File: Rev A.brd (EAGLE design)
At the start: 160 x 100 mm, 28 parts

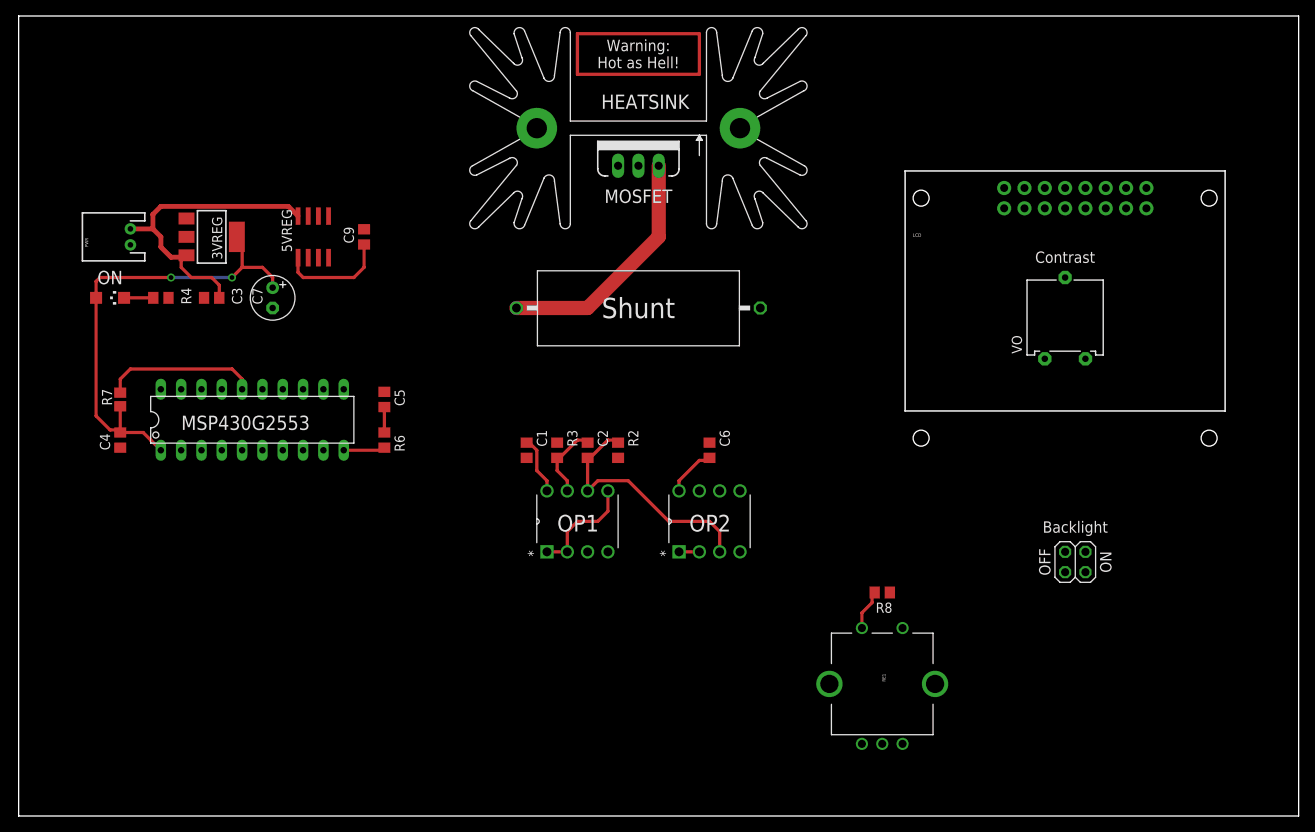
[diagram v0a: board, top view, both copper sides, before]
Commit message: Looks good to me
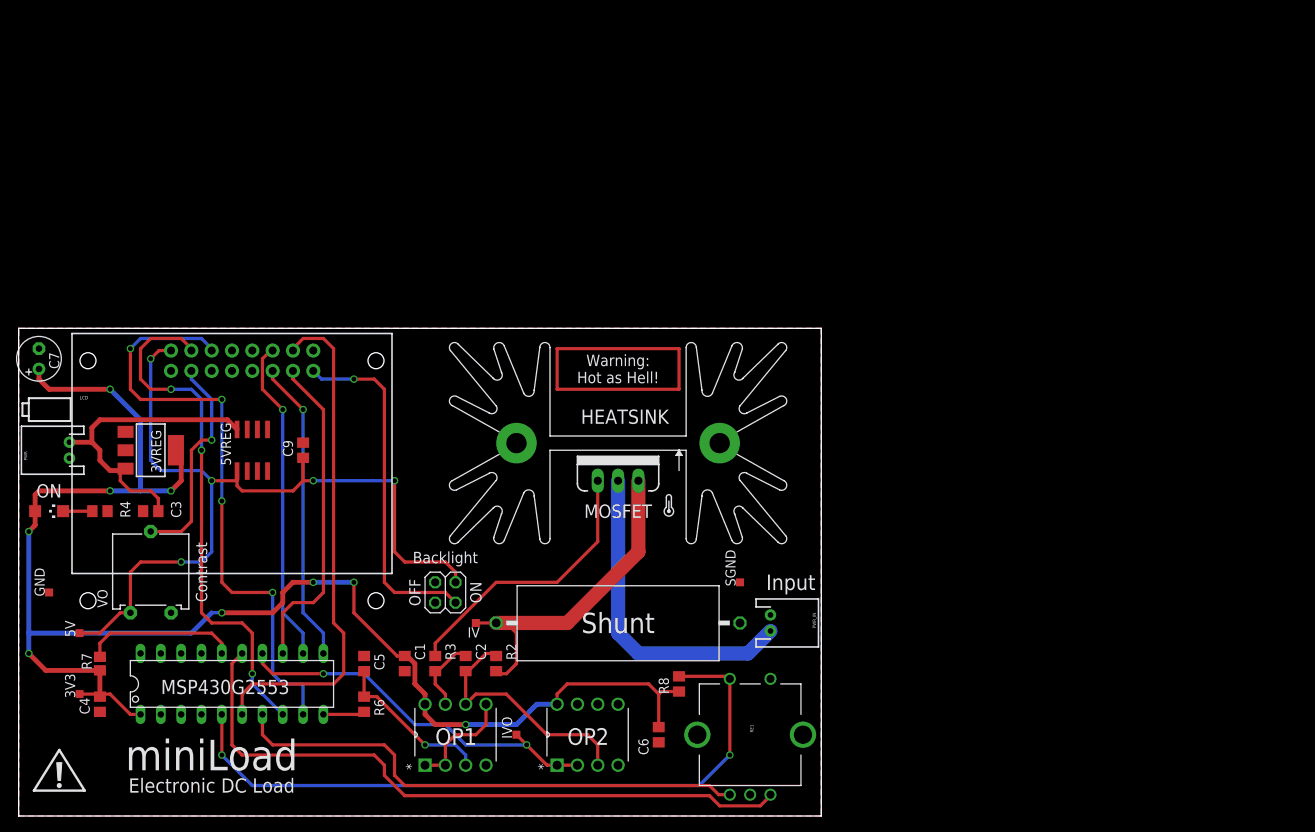
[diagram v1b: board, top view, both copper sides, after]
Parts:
- added 3V3, 5V, GND, IV, IVO, SGND: PTR1TP10SQ, testpad:TP10SQ
- added PWR_IN: M02JST-PTH-2, SparkFun-Connectors:JST-2-PTH
- added U$1: (no value), dicons:ICON_TEMP
- added U$2: (no value), dicons:ICON_EXL-S
- added U$3: (no value), dicons:ICON_BATTERY-S
- moved VO 118.6 mm to (16.5, 30.5)
- moved LCD 106.1 mm to (26.7, 41.9)
- moved JP_BKL 78.8 mm to (53.3, 27.9)
- moved HEATSINK 39.5 mm to (74.9, 45.7)
- moved N-CHANNEL 39.5 mm to (74.9, 41.9)
- moved SHUNT 39.5 mm to (74.9, 24.1)
- moved C6 36.1 mm to (80.0, 10.2), turned to 90 degrees
- moved C4 33.1 mm to (10.2, 14.0)
- moved R6 33.1 mm to (43.2, 14.0)
- moved C5 33.1 mm to (43.2, 19.1)
- moved MCU 33.1 mm to (26.7, 16.5)
- moved R7 33.1 mm to (10.2, 19.1)
- moved R2 30.7 mm to (59.7, 19.1)
- moved OP1 30.7 mm to (58.4, 14.0)
- moved OP2 30.7 mm to (74.9, 14.0)
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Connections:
- net +5V: now also 5V.TP
- net CURR_SENSE: now also IVO.TP
- net GND: now also GND.TP, PWR_IN.1, SGND.TP
- net N$13: now also IV.TP
- net TVIN: now also PWR_IN.2
- net VCC: now also 3V3.TP
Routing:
- net VCC: track 72.6 -> 195.5 mm, vias 2 -> 9
- net +5V: track 13.7 -> 104.1 mm, vias 0 -> 5
- net RE_B: track 0.00 -> 83.8 mm
- net RE_BTN: track 5.10 -> 87.7 mm, vias 0 -> 2
- net LCD_EN: track 0.00 -> 76.5 mm, vias 0 -> 4
- net RS: track 0.00 -> 65.9 mm, vias 0 -> 3
- net RE_A: track 0.00 -> 65.6 mm
- net DB7: track 0.00 -> 63.8 mm
- net CURR_SENSE: track 2.54 -> 47.7 mm, vias 0 -> 2
- net N$11: track 0.00 -> 43.9 mm, vias 0 -> 1
- net DB5: track 0.00 -> 40.6 mm, vias 0 -> 1
- net DB6: track 0.00 -> 40.5 mm
- net TVIN: track 0.00 -> 40.3 mm
- net DB4: track 0.00 -> 38.0 mm, vias 0 -> 1
- net N$3: track 0.00 -> 34.8 mm
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- added copper zone on layer 1, net GND
- added copper zone on layer 16, net GND
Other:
- board size 160 x 100 mm -> 100.3 x 61 mm
- board text added: "Electronic DC Load"
- board text added: "Input"
- board text added: "Nathan Campos, 2013"
- board text added: "miniLoad"
